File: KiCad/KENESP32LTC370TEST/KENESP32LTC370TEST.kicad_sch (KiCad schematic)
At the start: 23 parts, among them J1 Test Point 10x Header, U1 LTC3780EUH-TRPBF

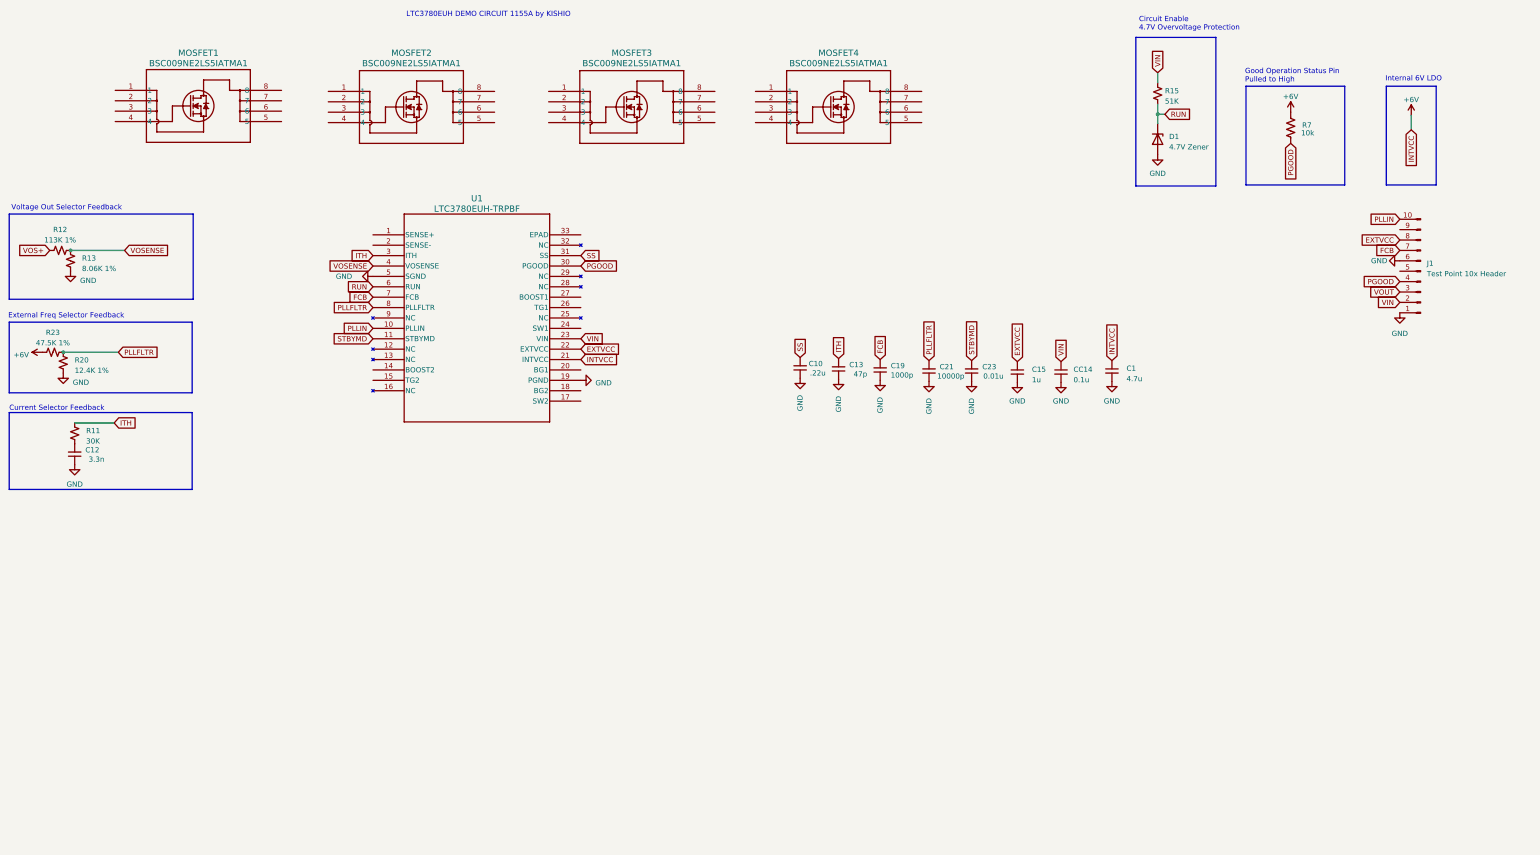
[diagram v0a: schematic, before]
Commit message: Finished Schematic
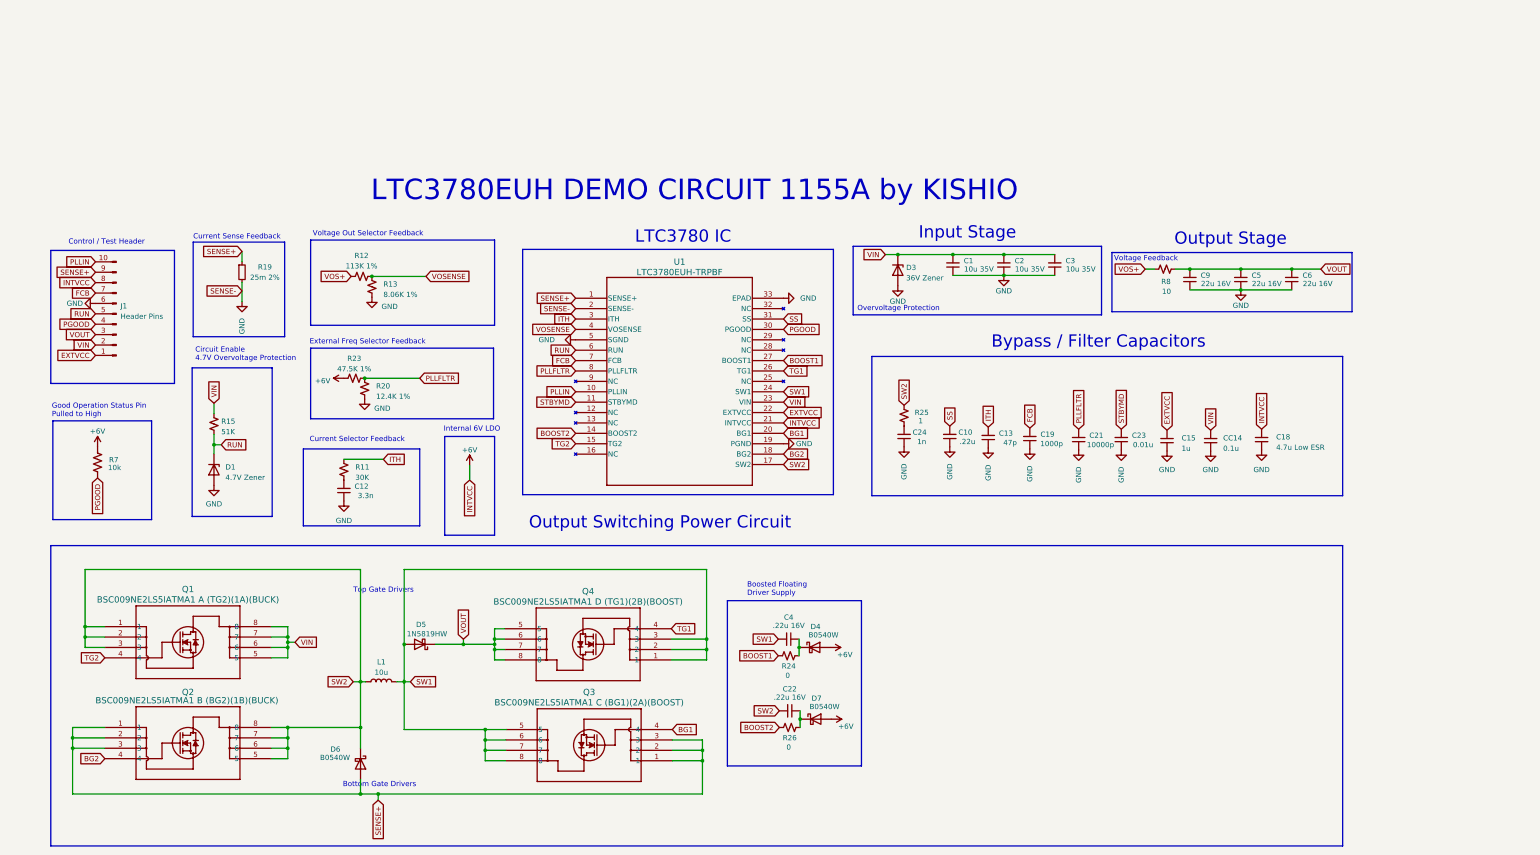
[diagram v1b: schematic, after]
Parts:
- added C1, C2, C3: 10u 35V, symbol Device:C_Small
- added C22, C4: .22u 16V, symbol Device:C_Small
- added C24: 1n, symbol Device:C_Small
- added C5, C6, C9: 22u 16V, symbol Device:C_Small
- added D3: 36V Zener, symbol Device:D_Zener
- added D4, D6, D7: B0540W, symbol Device:D_Schottky
- added D5: 1N5819HW, symbol Device:D_Schottky
- added L1: 10u, symbol Device:L
- added R19: 25m 2%, symbol Device:R_Small
- added R24, R26: 0, symbol Device:R_Small_US
- added R25: 1, symbol Device:R_Small_US
- added R8: 10, symbol Device:R_Small_US
- C18: renamed from C1; value 4.7u -> 4.7u Low ESR
- J1: value Test Point 10x Header -> Header Pins
- Q1: renamed from MOSFET1; value BSC009NE2LS5IATMA1 -> BSC009NE2LS5IATMA1 A (TG2)(1A)(BUCK)
- Q2: renamed from MOSFET2; value BSC009NE2LS5IATMA1 -> BSC009NE2LS5IATMA1 B (BG2)(1B)(BUCK)
- Q3: renamed from MOSFET3; value BSC009NE2LS5IATMA1 -> BSC009NE2LS5IATMA1 C (BG1)(2A)(BOOST)
- Q4: renamed from MOSFET4; value BSC009NE2LS5IATMA1 -> BSC009NE2LS5IATMA1 D (TG1)(2B)(BOOST)
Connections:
- net +6V: now also J1.8 (Pin_8), D4.2 (A), D7.2 (A)
- net EXTVCC: now also J1.1 (Pin_1); no longer J1.8 (Pin_8)
- net GND: now also U1.2 (SENSE-), U1.33 (EPAD), C1.1, C2.1, C24.1, C3.1, C5.1, C6.1, C9.1, D3.2 (A), R19.2; no longer J1.1 (Pin_1)
- net RUN: now also J1.5 (Pin_5)
- net VIN: now also Q1.5, Q1.6, Q1.7, Q1.8, C1.2, C2.2, C3.2, D3.1 (K)
- net VOS+: now also R8.2
- net VOUT: now also Q4.5, Q4.6, Q4.7, Q4.8, C5.2, C6.2, C9.2, D5.1 (K), R8.1
- net SW2: now reaches Q1.1
- net SW2: now also Q1.2, Q1.3, Q2.5, Q2.6, Q2.7, Q2.8, U1.17 (SW2), C22.2, D6.1 (K), L1.1, R25.2
- net TG2: now reaches Q1.4
- net TG2: now also U1.15 (TG2)
- net SENSE+: now reaches U1.1 (SENSE+)
- net SENSE+: now also J1.9 (Pin_9), Q2.1, Q2.2, Q2.3, Q3.1, Q3.2, Q3.3, D6.2 (A), R19.1
- net BOOST2: now reaches U1.14 (BOOST2)
- net BOOST2: now also R26.1
- net BG2: now reaches U1.18 (BG2)
- net BG2: now also Q2.4
- net BG1: now reaches U1.20 (BG1)
- net BG1: now also Q3.4
- net SW1: now reaches U1.24 (SW1)
- net SW1: now also Q3.5, Q3.6, Q3.7, Q3.8, Q4.1, Q4.2, Q4.3, C4.2, D5.2 (A), L1.2
- net TG1: now reaches U1.26 (TG1)
- net TG1: now also Q4.4
- net BOOST1: now reaches U1.27 (BOOST1)
- net BOOST1: now also R24.1
- new net: C22.1, D7.1 (K), R26.2
- new net: C4.1, D4.1 (K), R24.2
- new net: C24.2, R25.1
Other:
- note added: "Boosted Floating Driver Supply"
- note added: "Bottom Gate Drivers"
- note added: "Bypass / Filter Capacitors"
- note added: "Control / Test Header"
- note added: "Current Sense Feedback"
- note added: "Input Stage"
- note added: "LTC3780 IC"
- note added: "Output Stage"
- note added: "Output Switching Power Circuit"
- note added: "Overvoltage Protection"
- note added: "Top Gate Drivers"
- note added: "Voltage Feedback"
- title: (none) -> LTC3780 Development Circuit
- moved on the sheet: C10, C12, C13, C15, C18, C19, C21, C23, CC14, D1, J1, Q1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
